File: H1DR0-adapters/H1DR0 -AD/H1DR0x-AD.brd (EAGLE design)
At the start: 34.6 x 30 mm, 3 parts

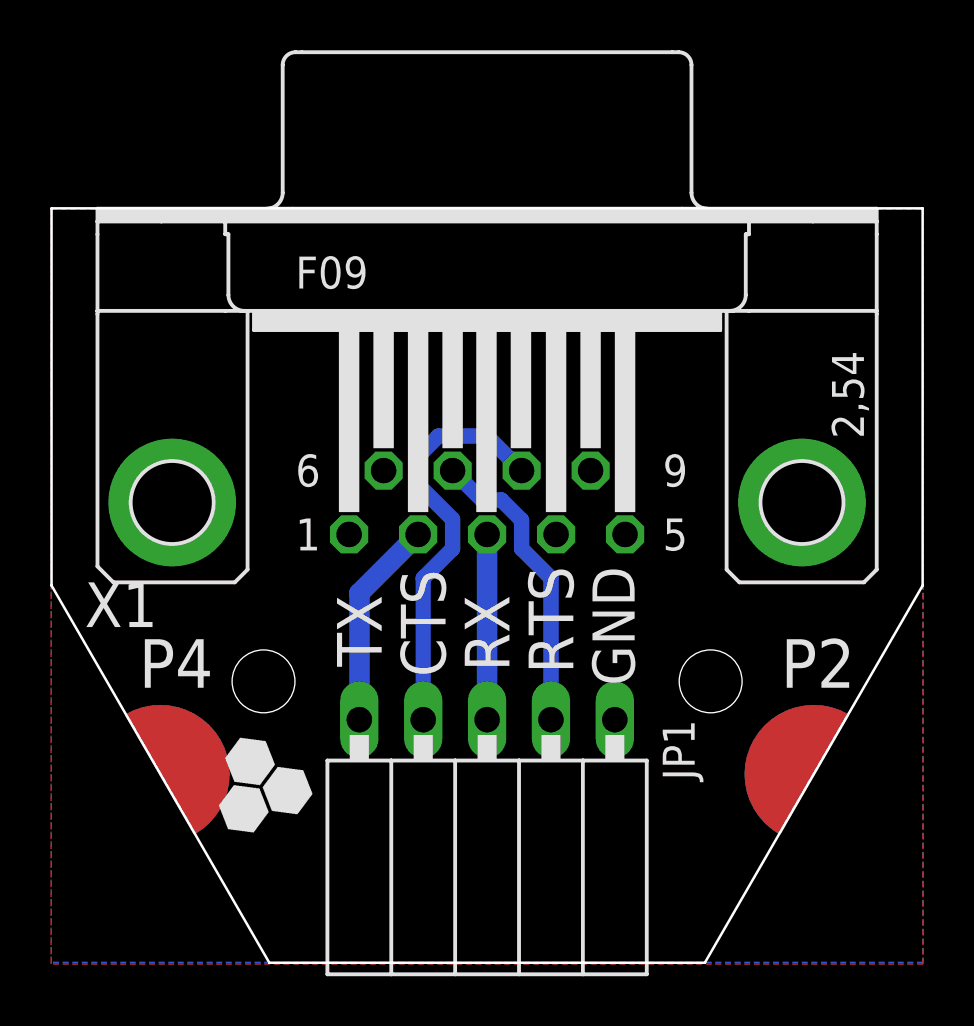
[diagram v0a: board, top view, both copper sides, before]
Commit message: no message
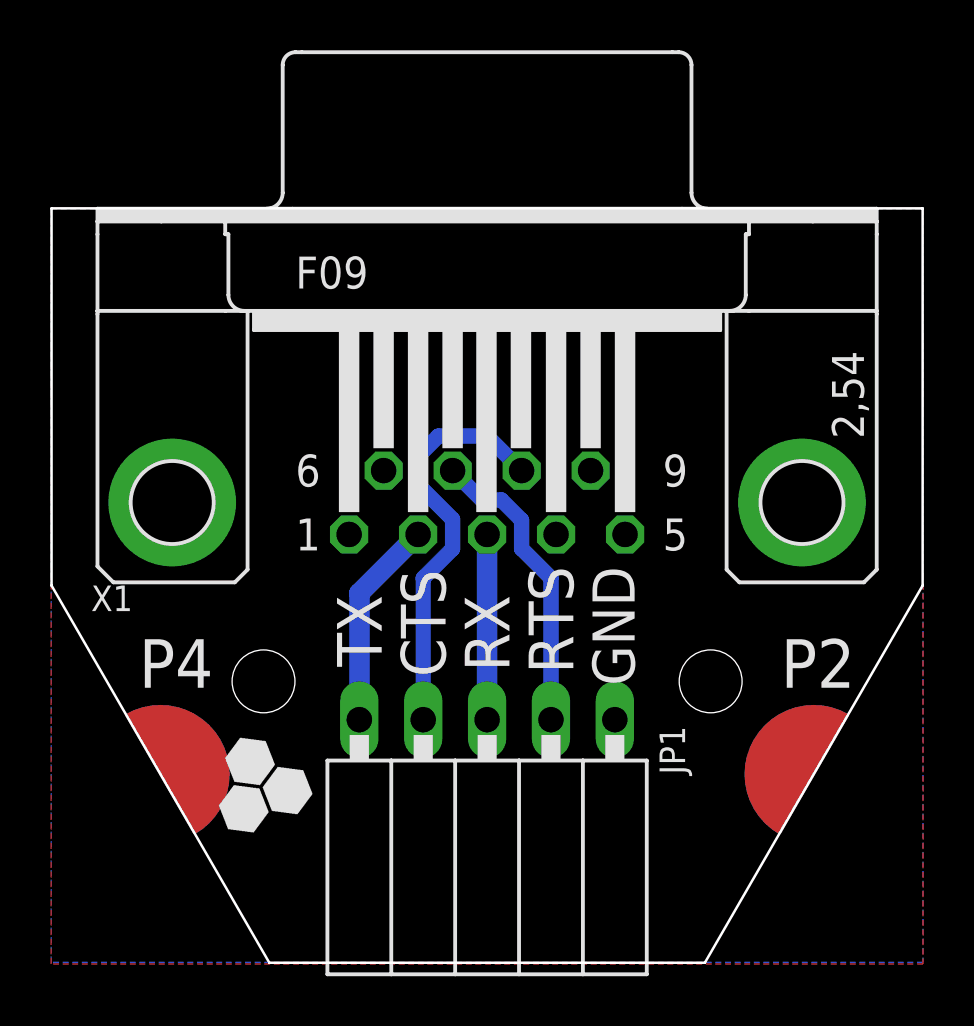
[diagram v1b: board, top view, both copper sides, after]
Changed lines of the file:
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@@
 <attribute name="MF" value="" x="47.117" y="10.922" size="1.778" layer="27" display="off"/>
 <attribute name="MPN" value="" x="47.117" y="10.922" size="1.778" layer="27" display="off"/>
-<attribute name="NAME" x="1.905" y="13.589" size="1.778" layer="25" ratio="10"/>
+<attribute name="NAME" x="2.159" y="14.224" size="1.016" layer="25" ratio="10"/>
 <attribute name="OC_FARNELL" value="unknown" x="47.117" y="10.922" size="1.778" layer="27" display="off"/>
 <attribute name="OC_NEWARK" value="unknown" x="47.117" y="10.922" size="1.778" layer="27" display="off"/>
@@
 <element name="U$1" library="hexabitz_connectors" package="HEXABIT_BUS_ADAPTER_WITH_P2_P4" value="HEXABIT_BUS_ADAPTER_WITH_PD2_PD4_PD9_PD10" x="17.907" y="15.24" smashed="yes"/>
 <element name="JP1" library="Hexabitz" package="F_1X05" value="" x="17.907" y="7.366" smashed="yes" rot="R180">
-<attribute name="NAME" x="24.892" y="9.906" size="1.27" layer="25" ratio="10" rot="R270"/>
+<attribute name="NAME" x="24.765" y="9.652" size="1.016" layer="25" ratio="10" rot="R270"/>
 <attribute name="VALUE" x="9.652" y="9.906" size="1.27" layer="27" rot="R270"/>
 </element>
